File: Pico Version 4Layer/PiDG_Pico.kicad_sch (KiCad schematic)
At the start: 43 parts, among them J1 Conn_02x05_Odd_Even, J10 Trig, J11 Laser Enable, J12 Pixel Reset, J14 Pico Socket A, J15 Pico Socket B, J16 Laser En/PWM Trig/GND, J2 Conn_02x05_Odd_Even, J3 Conn_02x05_Odd_Even, J4 Conn_02x05_Odd_Even, J5 Conn_02x05_Odd_Even, J6 Conn_02x05_Odd_Even, J7 Laser 1, J8 Laser 2, U1 74LVC1G04, U10 74LVC1G08, U11 Raspberry Pi Pico 2 W, U12 74LVC1G08, U13 UCC27524, U2 SN74LVC04AD, U3 74LVC1G04, U4 SN74LVC04AD, U5 74LVC1G04, U6 SN74LVC04AD, U7 74LVC1G08, U8 74LVC1G08

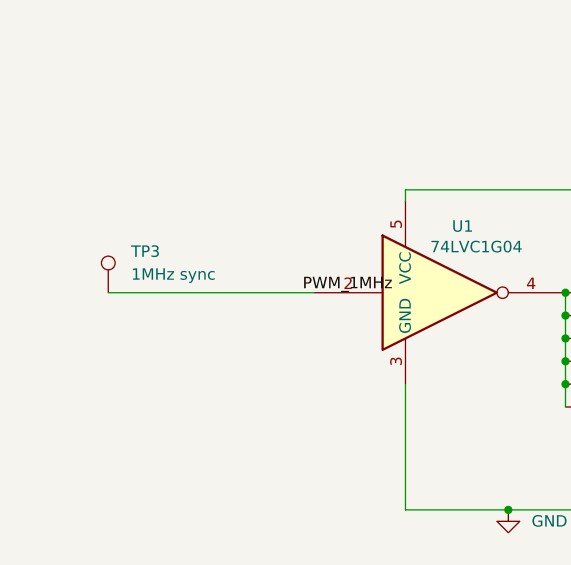
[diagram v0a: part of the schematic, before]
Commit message: Refined and ready version
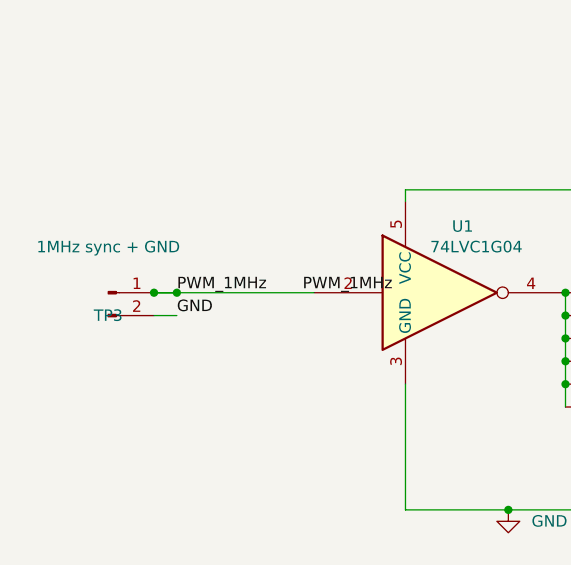
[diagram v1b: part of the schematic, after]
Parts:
- removed TP3: 1MHz sync, Connector_PinHeader_2.54mm:PinHeader_1x01_P2.54mm_Horizontal, symbol Connector:TestPoint
- added TP3: 1MHz sync + GND, Connector_PinHeader_2.54mm:PinHeader_1x02_P2.54mm_Horizontal, symbol Connector:Conn_01x02_Pin
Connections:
- net GND: now also TP3.2 (Pin_2)
- net PWM_1MHz: now also TP3.1 (Pin_1)
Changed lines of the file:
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@@
 	(wire
 		(pts
-			(xy 21.59 43.18) (xy 44.45 43.18)
+			(xy 26.67 43.18) (xy 29.21 43.18)
+		)
+		(stroke
+			(width 0)
+			(type default)
+		)
+	)
+	(wire
+		(pts
+			(xy 29.21 43.18) (xy 44.45 43.18)
 		)
 		(stroke
@@
 	)
 	(symbol
-		(lib_id "Connector:TestPoint")
-		(at 21.59 43.18 0)
-		(unit 1)
-		(body_style 1)
-		(exclude_from_sim no)
-		(in_bom yes)
-		(on_board yes)
-		(in_pos_files yes)
-		(dnp no)
-		(fields_autoplaced yes)
-		(property "Reference" "TP3"
-			(at 24.13 38.6079 0)
-			(show_name no)
-			(do_not_autoplace no)
-			(effects
-				(font
-					(size 1.27 1.27)
-				)
-				(justify left)
-			)
-		)
-		(property "Value" "1MHz sync"
-			(at 24.13 41.1479 0)
-			(show_name no)
-			(do_not_autoplace no)
-			(effects
-				(font
-					(size 1.27 1.27)
-				)
-				(justify left)
-			)
-		)
-		(property "Footprint" "Connector_PinHeader_2.54mm:PinHeader_1x01_P2.54mm_Horizontal"
-			(at 26.67 43.18 0)
-			(hide yes)
-			(show_name no)
-			(do_not_autoplace no)
-			(effects
-				(font
-					(size 1.27 1.27)
-				)
-			)
-		)
-		(property "Datasheet" ""
-			(at 26.67 43.18 0)
-			(hide yes)
-			(show_name no)
-			(do_not_autoplace no)
-			(effects
-				(font
-					(size 1.27 1.27)
-				)
-			)
-		)
-		(property "Description" "test point"
-			(at 21.59 43.18 0)
-			(hide yes)
-			(show_name no)
-			(do_not_autoplace no)
-			(effects
-				(font
-					(size 1.27 1.27)
-				)
-			)
-		)
-		(pin "1"
-		)
-		(instances
-			(project "PiDG_Pico"
-				(path "/e63e39d7-6ac0-4ffd-8aa3-1841a4541b55"
-					(reference "TP3")
-					(unit 1)
-				)
-			)
-		)
-	)
-	(symbol
 		(lib_id "power:GND")
 		(at 50.8 241.3 0)
@@
 		)
 	)
+	(symbol
+		(lib_id "Connector:Conn_01x02_Pin")
+		(at 21.59 43.18 0)
+		(unit 1)
+		(body_style 1)
+		(exclude_from_sim no)
+		(in_bom yes)
+		(on_board yes)
+		(in_pos_files yes)
+		(dnp no)
+		(property "Reference" "TP3"
+			(at 21.59 45.72 0)
+			(show_name no)
+			(do_not_autoplace no)
+			(effects
+				(font
+					(size 1.27 1.27)
+				)
+			)
+		)
+		(property "Value" "1MHz sync + GND"
+			(at 21.59 38.1 0)
+			(show_name no)
+			(do_not_autoplace no)
+			(effects
+				(font
+					(size 1.27 1.27)
+				)
+			)
+		)
+		(property "Footprint" "Connector_PinHeader_2.54mm:PinHeader_1x02_P2.54mm_Horizontal"
+			(at 21.59 43.18 0)
+			(hide yes)
+			(show_name no)
+			(do_not_autoplace no)
+			(effects
+				(font
+					(size 1.27 1.27)
+				)
+			)
+		)
+		(property "Datasheet" ""
+			(at 21.59 43.18 0)
+			(hide yes)
+			(show_name no)
+			(do_not_autoplace no)
+			(effects
+				(font
+					(size 1.27 1.27)
+				)
+			)
+		)
+		(property "Description" "test point"
+			(at 21.59 43.18 0)
+			(hide yes)
+			(show_name no)
+			(do_not_autoplace no)
+			(effects
+				(font
+					(size 1.27 1.27)
+				)
+			)
+		)
+		(pin "1"
+		)
+		(pin "2"
+		)
+		(instances
+			(project "PiDG_Pico"
+				(path "/e63e39d7-6ac0-4ffd-8aa3-1841a4541b55"
+					(reference "TP3")
+					(unit 1)
+				)
+			)
+		)
+	)
+	(wire
+		(pts
+			(xy 26.67 43.18) (xy 29.21 43.18)
+		)
+		(stroke
+			(width 0)
+			(type default)
+		)
+	)
+	(junction
+		(at 26.67 43.18)
+		(diameter 0)
+		(color 0 0 0 0)
+	)
+	(junction
+		(at 29.21 43.18)
+		(diameter 0)
+		(color 0 0 0 0)
+	)
+	(label "PWM_1MHz"
+		(at 29.21 43.18 0)
+		(effects
+			(font
+				(size 1.27 1.27)
+			)
+			(justify left bottom)
+		)
+	)
+	(wire
+		(pts
+			(xy 26.67 45.72) (xy 29.21 45.72)
+		)
+		(stroke
+			(width 0)
+			(type default)
+		)
+	)
+	(label "GND"
+		(at 29.21 45.72 0)
+		(effects
+			(font
+				(size 1.27 1.27)
+			)
+			(justify left bottom)
+		)
+	)
